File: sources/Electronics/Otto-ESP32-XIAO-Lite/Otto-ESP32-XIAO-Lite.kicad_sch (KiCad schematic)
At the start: 20 parts, among them J1 Conn_01x03, J10 Conn_01x02, J12 OLED 0,91" - I2C (SKU21796), J13 MPU6050, J2 Conn_01x03, J3 Conn_01x03, J4 Conn_01x03, J5 Conn_01x03, J6 Conn_01x03, J7 Ultrasonic sensor, J8 PCA9685, SW1 SW_SPDT, U1 MOUDLE-SEEEDUINO-XIAO-ESP32C3, U2 R-78E5.0-1.0

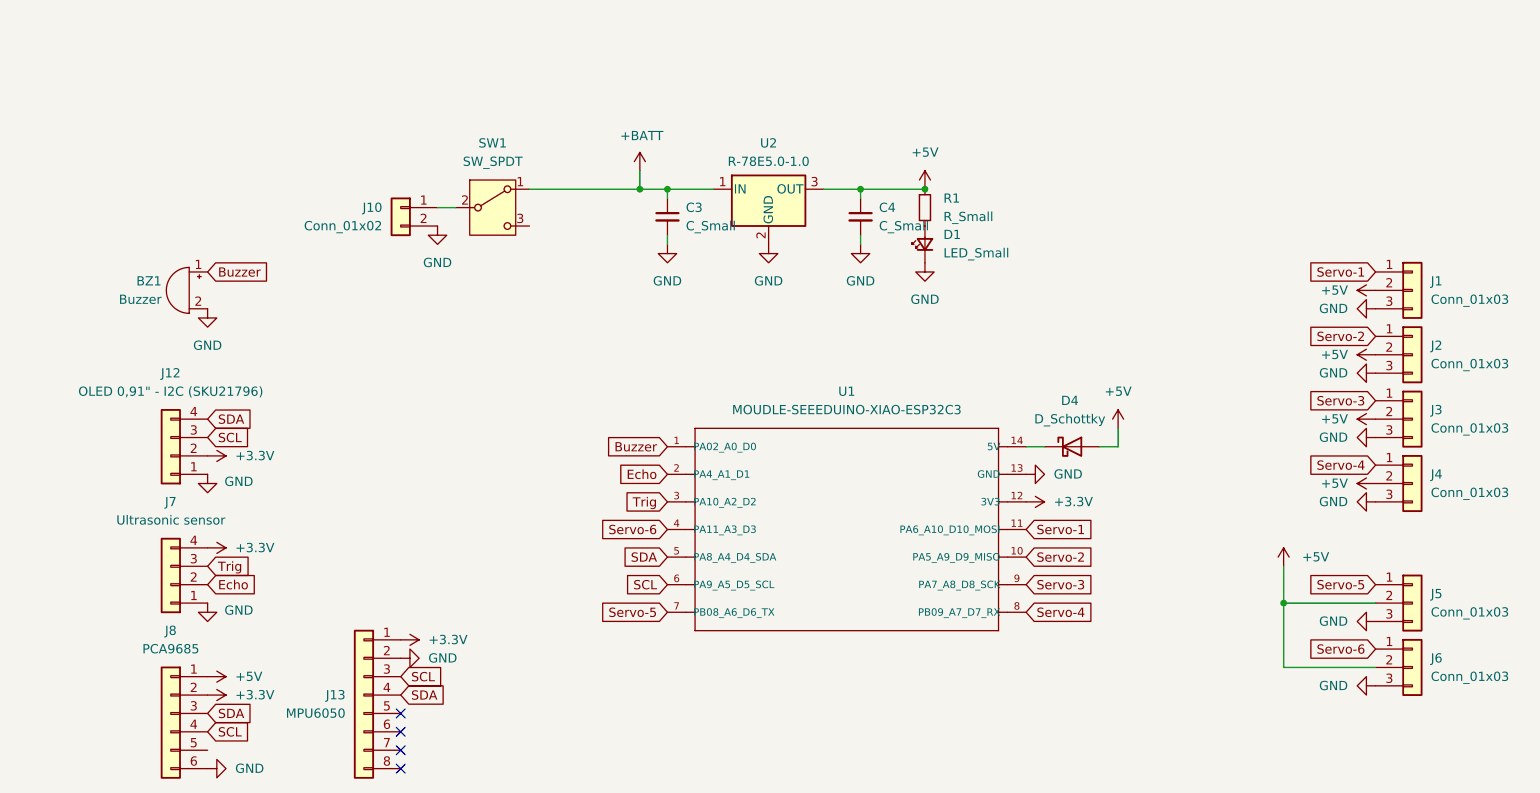
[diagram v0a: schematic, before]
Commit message: update documentation
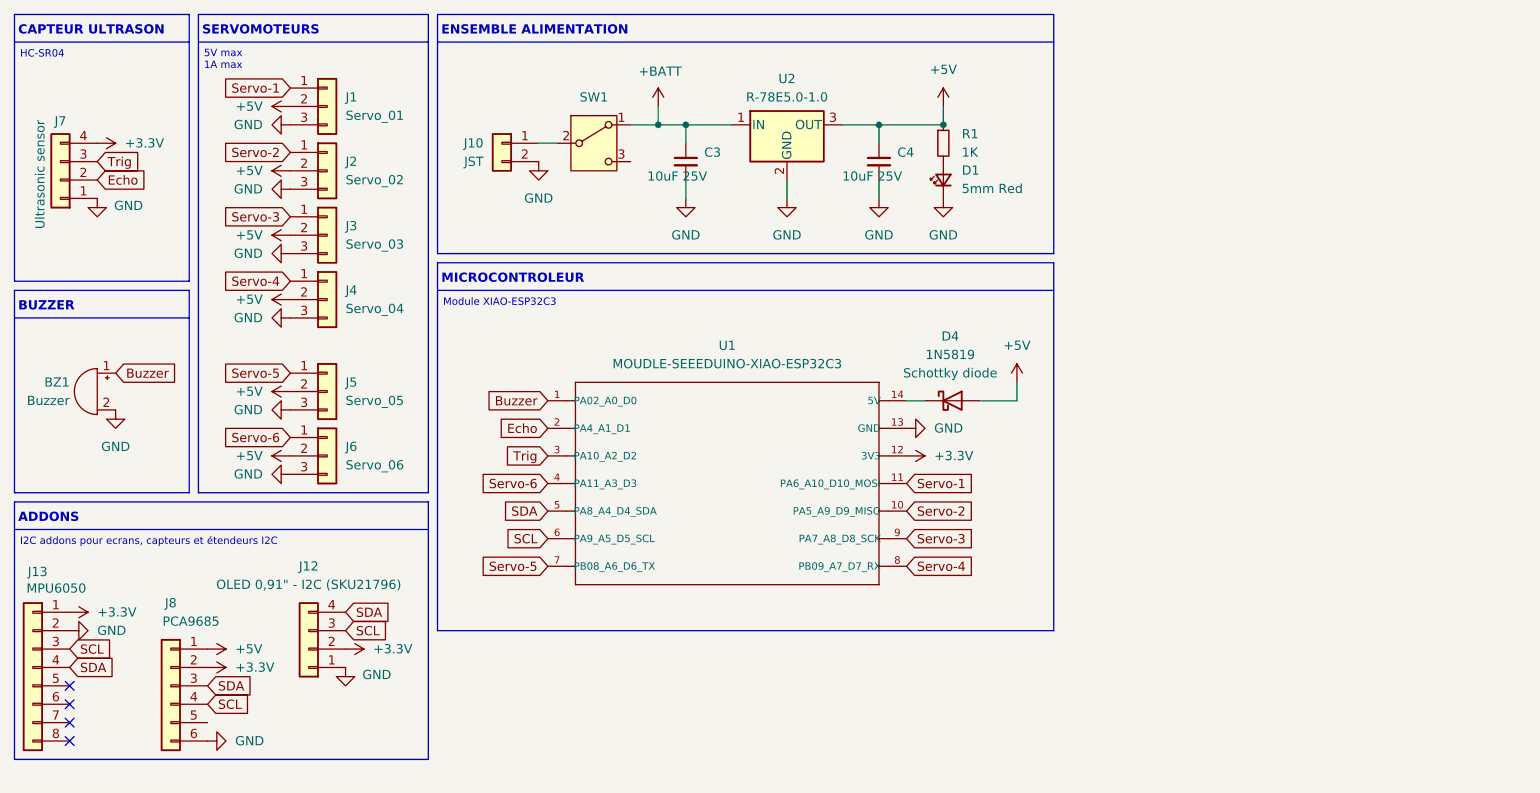
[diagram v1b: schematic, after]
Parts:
- C3, C4: value C_Small -> 10uF 25V
- D1: value LED_Small -> 5mm Red
- D4: value D_Schottky -> 1N5819
- J1: value Conn_01x03 -> Servo_01
- J10: value Conn_01x02 -> JST
- J2: value Conn_01x03 -> Servo_02
- J3: value Conn_01x03 -> Servo_03
- J4: value Conn_01x03 -> Servo_04
- J5: value Conn_01x03 -> Servo_05
- J6: value Conn_01x03 -> Servo_06
- R1: value R_Small -> 1K
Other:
- note added: "5V max 1A max"
- note added: "ADDONS"
- note added: "BUZZER"
- note added: "CAPTEUR ULTRASON"
- note added: "ENSEMBLE ALIMENTATION"
- note added: "HC-SR04"
- note added: "I2C addons pour ecrans, capteurs et étendeurs I2C"
- note added: "MICROCONTROLEUR"
- note added: "Module XIAO-ESP32C3"
- note added: "SERVOMOTEURS"
- company: (none) -> UniLaSalle Amiens - MakerSpace
- title: (none) -> PCB Otto Mks
- moved on the sheet: BZ1, C3, C4, D1, D4, J1, J10, J12, J13, J2, J3, J4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
